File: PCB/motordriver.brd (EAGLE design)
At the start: 100 x 80 mm, 46 parts, among them IC1 7818TV

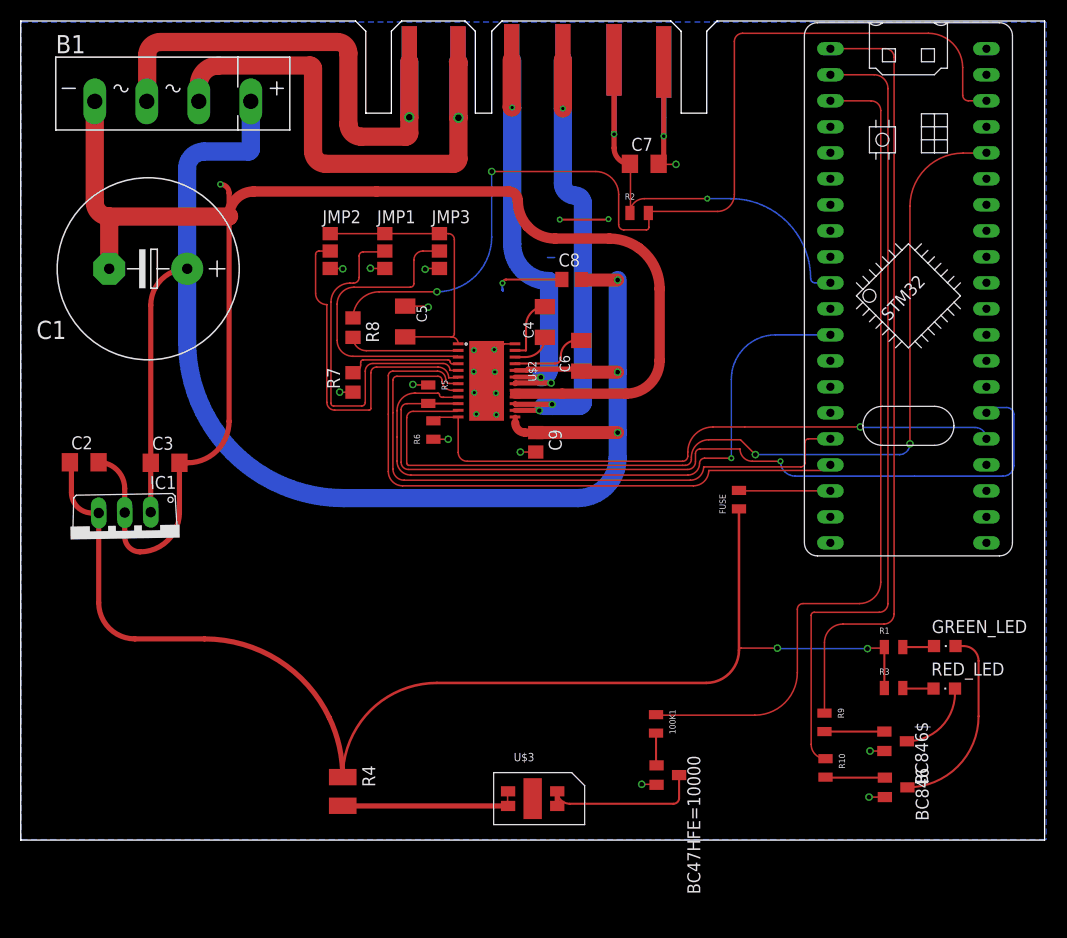
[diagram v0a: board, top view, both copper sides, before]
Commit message: PCB/motordriver.sch
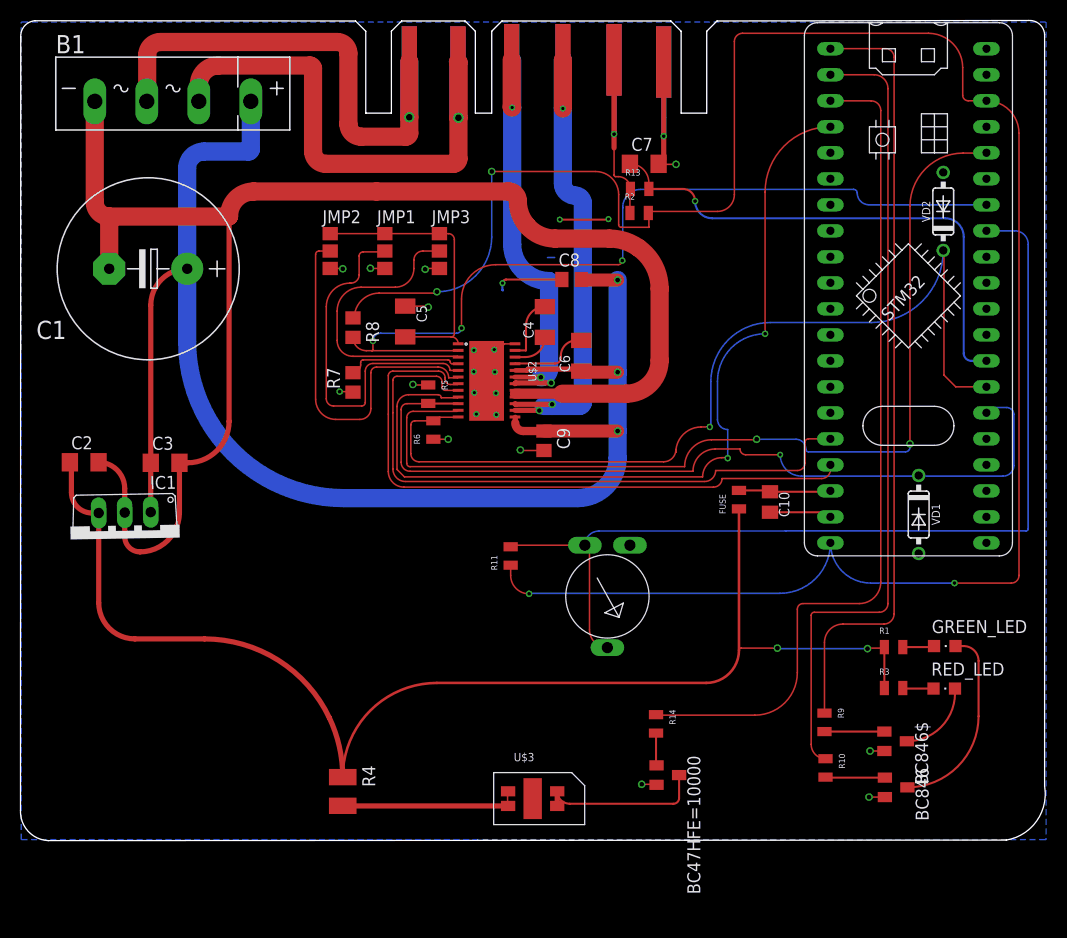
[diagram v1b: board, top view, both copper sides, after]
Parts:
- removed OUT, OUT1, OUT2, OUT3: SMDPAD, myLibrary:1.5X7MMPAD
- added C10: (no value), rcl:C0805K
- added OUT1_JMP_A, OUT1_JMP_B, OUT2_JMP_A, OUT2_JMP_B: SMDPAD, myLibrary:1.5X7MMPAD
- added R11: 10k, myLibrary:0805
- added R12: 10k, myLibrary:3X1MM
- added R13: 160, myLibrary:0805
- added VD1, VD2: 3.3V, zener:DO35-7
- moved C9 0.81 mm to (51.1, 39.0)
- renumbered 100K1 to R14
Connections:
- removed net N$12: OUT1.P$1, OUT3.P$1, U$2.14, U$2.15
- removed net N$13: OUT.P$1, OUT2.P$1, U$2.18, U$2.19
- removed net TOARM: R8.2, U$2.2
- new net B: IN1.P$1, IN3.P$1, R13.P$1, R2.P$1
- new net OUT1: OUT1_JMP_A.P$1, OUT1_JMP_B.P$1, U$2.18, U$2.19
- new net OUT2: OUT2_JMP_A.P$1, OUT2_JMP_B.P$1, U$2.14, U$2.15
- new net PA10: U$1.P$7
- new net PA11: U$1.P$8
- new net PA12: U$1.P$9
- new net PA2: R6.P$2, U$1.P$34, U$2.12, VD2.C
- new net PA3: C7.1, R13.P$2, U$1.P$33
- new net PA4: U$1.P$32
- new net PA5: U$1.P$31
- new net PA6: U$1.P$30
- new net PA7: U$1.P$29
- new net PA8: U$1.P$5
- new net PA9: U$1.P$6
- new net PB1: R8.2, U$1.P$27, U$2.2
- new net PB10: U$1.P$26
- new net PB15: U$1.P$4, U$2.9
- new net PB5: U$1.P$13
- new net PB6: U$1.P$14
- new net PB7: U$1.P$15
- new net PC13: U$1.P$39
- new net PC14: U$1.P$38
- new net PC15: U$1.P$37
- net 3.3V: now also R11.P$1
- net GND: now also C10.2, R12.-, VD1.A, VD2.A
- net N$26: now also C10.1
- net PA0: no longer R6.P$2, U$2.12
- net PA1: now also VD1.C
- net PA15: no longer C7.1, IN1.P$1, IN3.P$1, R2.P$1
- net PB0: now also R11.P$2, R12.+, R12.FLOATING
- net PB4: no longer U$2.9
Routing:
- net 3.3V: track 97.6 -> 200.4 mm, vias 2 -> 4
- net PB0: track 0.00 -> 94.6 mm
- net PA2: track 0.00 -> 88.3 mm, vias 0 -> 1
- net PB15: track 0.00 -> 83.5 mm, vias 0 -> 2
- net PB1: track 0.00 -> 83.5 mm, vias 0 -> 3
- net PB4: track 65.0 -> 0.00 mm, vias 1 -> 0
- net PA0: track 60.1 -> 0.00 mm, vias 1 -> 0
- net OUT2: track 0.00 -> 49.8 mm, vias 0 -> 3
- net N$12: track 49.8 -> 0.00 mm, vias 3 -> 0
- net PA3: track 0.00 -> 49.8 mm, vias 0 -> 1
- net PA15: track 46.5 -> 0.00 mm, vias 2 -> 0
- net OUT1: track 0.00 -> 44.8 mm, vias 0 -> 3
- net N$13: track 44.8 -> 0.00 mm, vias 3 -> 0
- net B: track 0.00 -> 23.0 mm, vias 0 -> 1
- net GND: track 248.6 -> 227.7 mm, vias 25 -> 24
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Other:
- board size 100 x 80 mm -> 100.1 x 80.1 mm
- board text added: "3.3V"
- board text added: "C1"
- board text added: "C10"
- board text added: "C2"
- board text added: "C3"
- board text added: "C4"
- board text added: "C5"
- board text added: "C6"
- board text added: "C7"
- board text added: "C8"
- board text added: "C9"
- board text added: "ERROR"
- board text added: "FUSE"
- board text added: "IC1"
- board text added: "LED"
- board text added: "MODE"
- board text added: "Max"
- board text added: "Min"
- board text added: "NOL"
- board text added: "R1"
- board text added: "R10"
- board text added: "R11"
- board text added: "R13"
- board text added: "R14"
- board text added: "R2"
- board text added: "R3"
- board text added: "R4"
- board text added: "R5"
- board text added: "R6"
- board text added: "R7"
- board text added: "R8"
- board text added: "R9"
- board text added: "SPEED"
- board text added: "STATUS"
- board text added: "T1"
- board text added: "T2"
- board text added: "T3"
- board text added: "drv"
- board text added: "nTRIP"
